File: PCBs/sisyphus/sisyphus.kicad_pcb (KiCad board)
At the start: 2 copper layers, 52 x 42 mm, 72 parts, among them J1 Light sensor, J10 Keyboard, J2 USB_C_Receptacle_USB2.0_14P, J3 AUX USB, J4 Conn_01x02, J5 Speaker, J6 Battery, J7 SWD, J8 Limit SW, J9 RGB_CONN, Q1 FS8205, U1 TPS62293, U2 USBLC6-2P6, U3 BQ25619, U4 W25Q128JVS, U5 MAX98357A, U6 DW01A, U7 RP2040, Y1 ABM8-272-T3

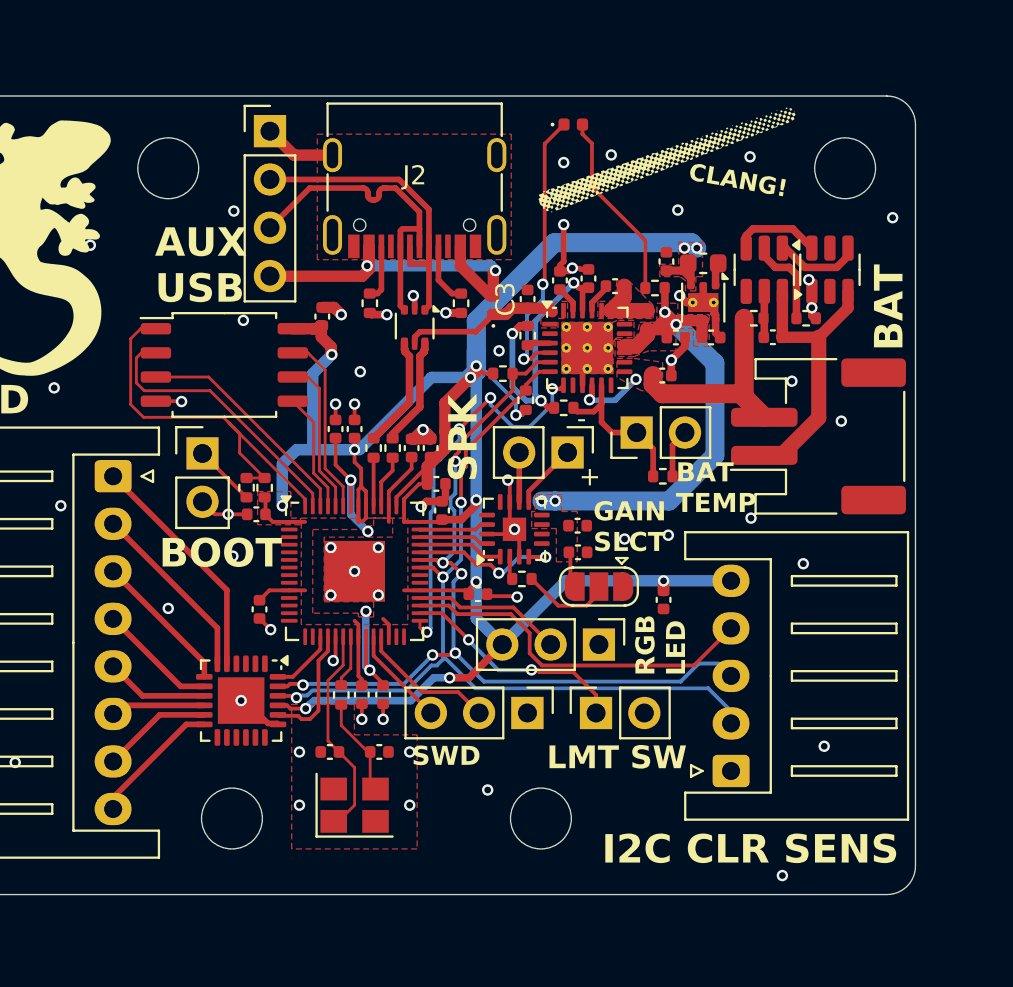
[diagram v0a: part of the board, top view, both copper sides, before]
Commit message: Add some ✨flair✨ to the PCB
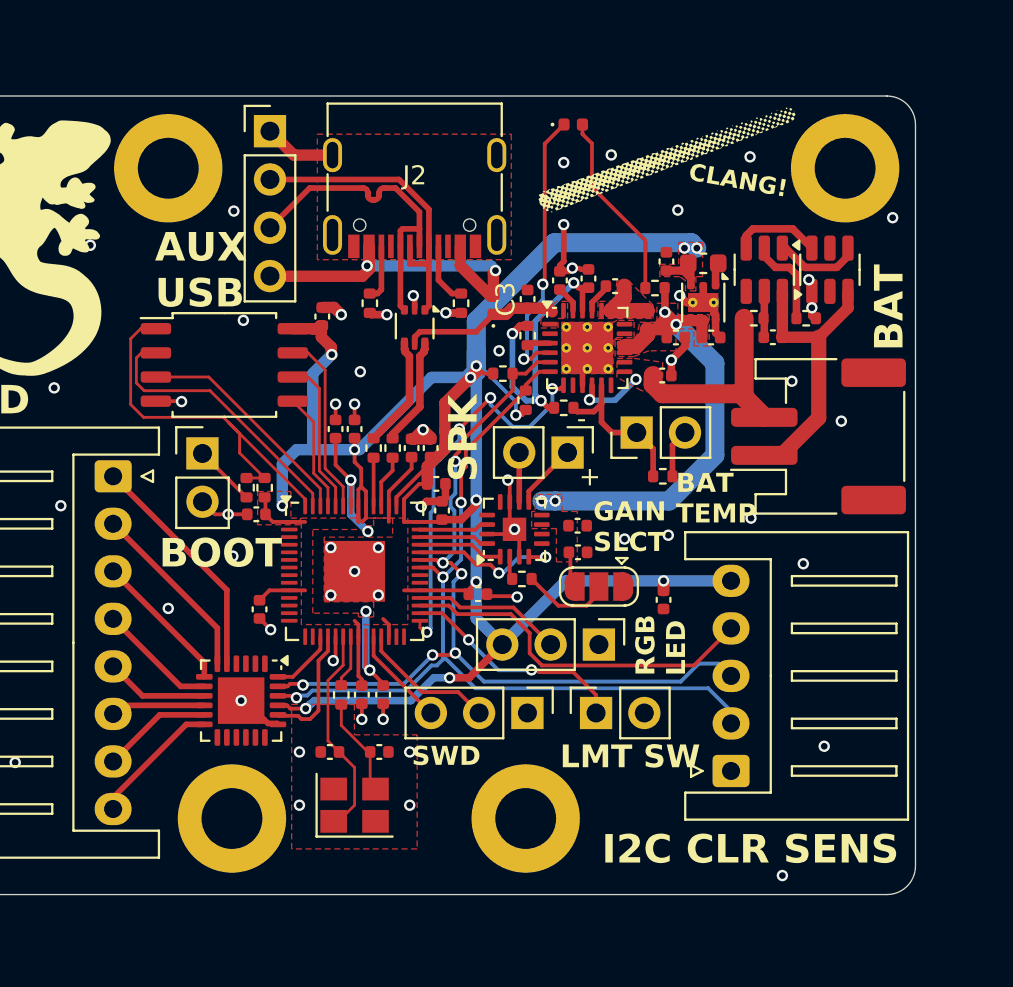
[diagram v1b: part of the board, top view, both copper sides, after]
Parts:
- H1, H2, H3, H4: footprint MountingHole:MountingHole_3.2mm_M3_ISO7380 -> MountingHole:MountingHole_3.2mm_M3_ISO7380_Pad
- moved H2 39.4 mm to (90.2, 78.8)
- moved H4 38.1 mm to (109.0, 113.0)
- moved H1 35.6 mm to (125.8, 78.8)
- moved H3 0.10 mm to (93.5, 113.0)
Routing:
- net GND: vias 57 -> 56
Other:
- board text added: "Ano, prosím"
- board text added: "Ještě víc!"
- board text added: "SisyFOSS"
- board text removed: "Ano, prosím, ještě víc!"
- board text removed: "SisypFOSS"
